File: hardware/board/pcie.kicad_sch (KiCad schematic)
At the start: 60 parts, among them CN2 1-2199230-5, U46 PI6C557-03BLE, U50 TP5108E23E-33, U51 SY8089AAAC, X6 X322525MOB4SI

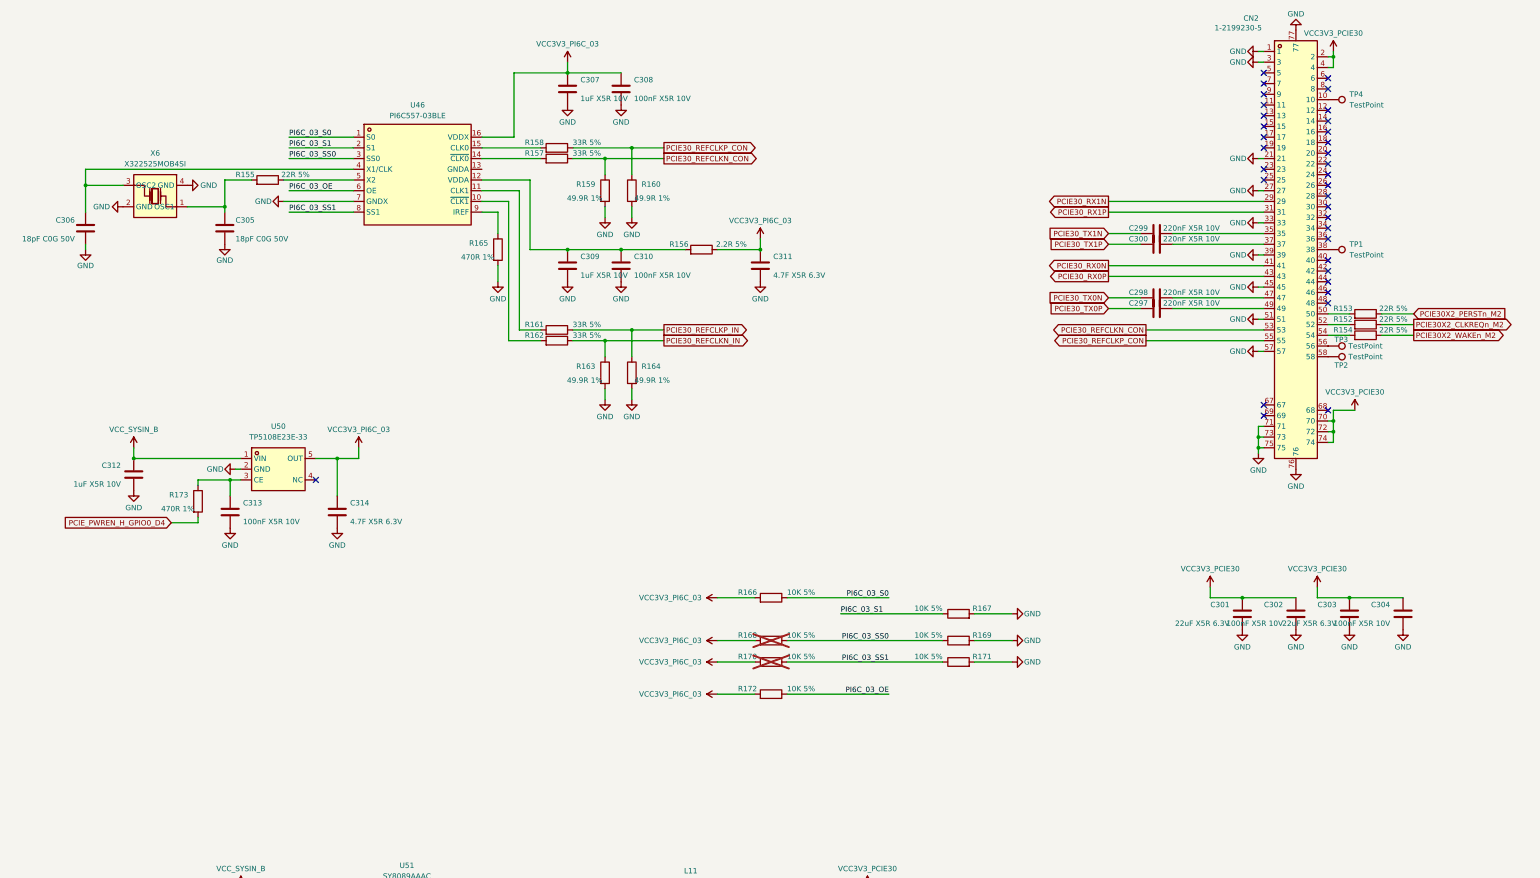
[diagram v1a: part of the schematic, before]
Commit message: finished schematic!
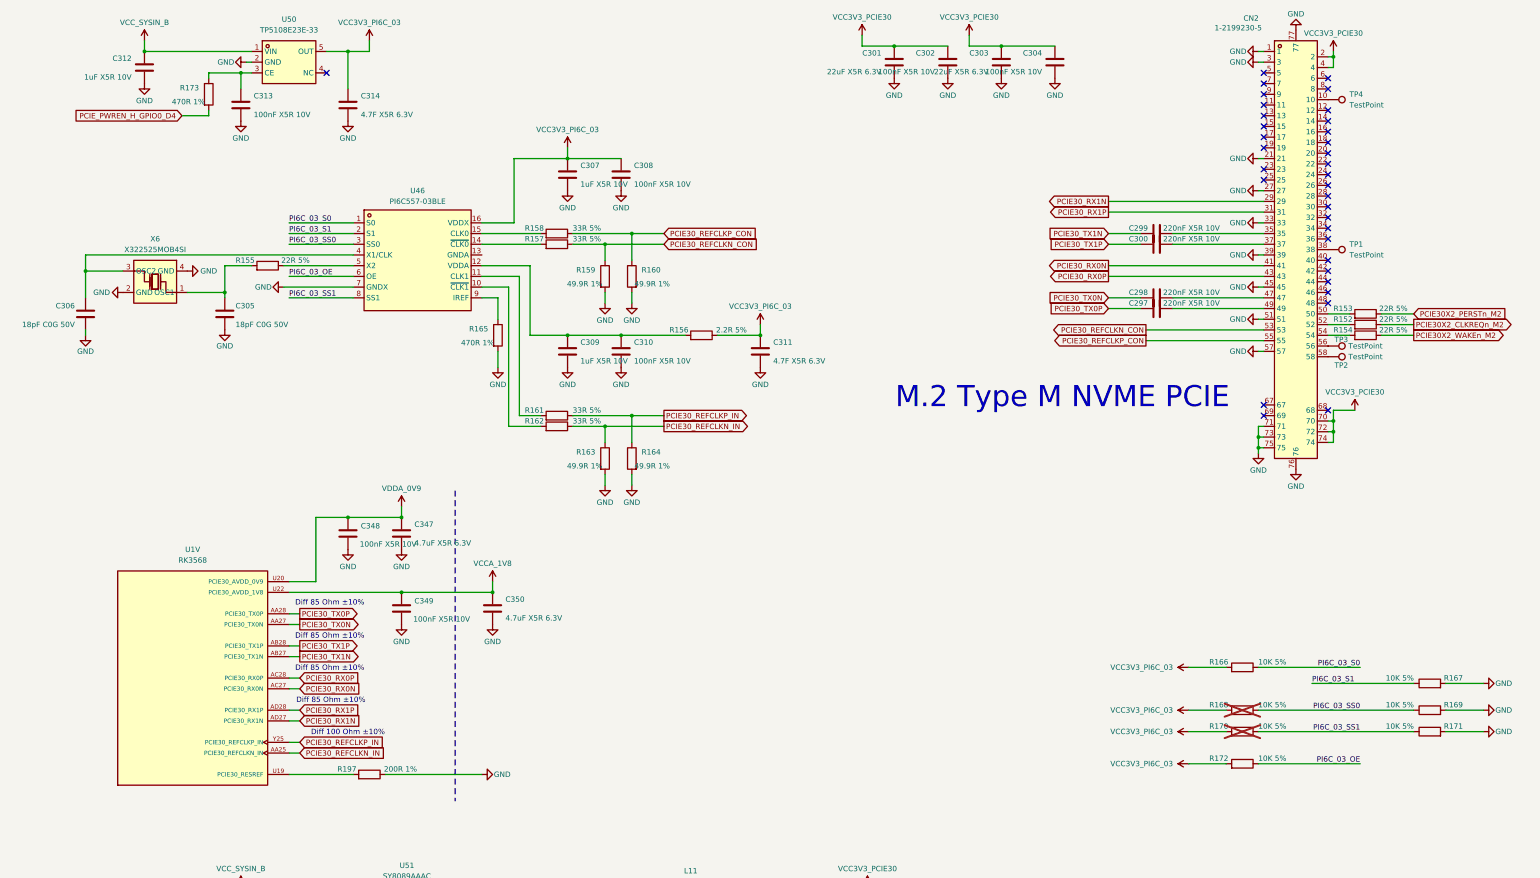
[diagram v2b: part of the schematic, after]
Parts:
- added C347, C350: 4.7uF X5R 6.3V, Capacitor_SMD:C_0402_1005Metric, symbol Device:C
- added C348, C349: 100nF X5R 10V, Capacitor_SMD:C_0201_0603Metric, symbol Device:C
- added R197: 200R 1%, Resistor_SMD:R_0201_0603Metric, symbol Device:R
- added U1: RK3568, RK3568:BGA636C65P28X28_1900X1900X168, symbol RK3568:RK3568
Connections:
- net GND: now also C347.2, C348.2, C349.2, C350.2, R197.1
- net PCIE30_REFCLKN_IN: now also U1.AA25 (PCIE30_REFCLKN_IN)
- net PCIE30_REFCLKP_IN: now also U1.Y25 (PCIE30_REFCLKP_IN)
- net PCIE30_RX0N: now also U1.AC27 (PCIE30_RX0N)
- net PCIE30_RX0P: now also U1.AC28 (PCIE30_RX0P)
- net PCIE30_RX1N: now also U1.AD27 (PCIE30_RX1N)
- net PCIE30_RX1P: now also U1.AD28 (PCIE30_RX1P)
- net PCIE30_TX0N: now also U1.AA27 (PCIE30_TX0N)
- net PCIE30_TX0P: now also U1.AA28 (PCIE30_TX0P)
- net PCIE30_TX1N: now also U1.AB27 (PCIE30_TX1N)
- net PCIE30_TX1P: now also U1.AB28 (PCIE30_TX1P)
- new net: R197.2, U1.U19 (PCIE30_RESREF)
- new net PCIE30_AVDD_0V9: C347.1, C348.1, U1.U20 (PCIE30_AVDD_0V9), U1.U21 (PCIE30_AVDD_0V9)
- new net VCCA_1V8: C349.1, C350.1, U1.U22 (PCIE30_AVDD_1V8)
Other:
- note added: "Diff 100 Ohm ±10%"
- note added: "Diff 85 Ohm ±10%"
- note added: "M.2 Type M NVME PCIE"
- moved on the sheet: C301, C302, C303, C304, C305, C306, C307, C308, C309, C310, C311, C312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

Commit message: finished beautifying schematic
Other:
- note added: "Clock Generator"
- note added: "Frost"
- note added: "M.2 Type B"
- note added: "Power / Decoupling"
- note added: "RK3568"
- note removed: "M.2 Type M NVME PCIE"
- moved on the sheet: C301, C302, C303, C304, C305, C306, C307, C308, C309, C310, C311, C312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

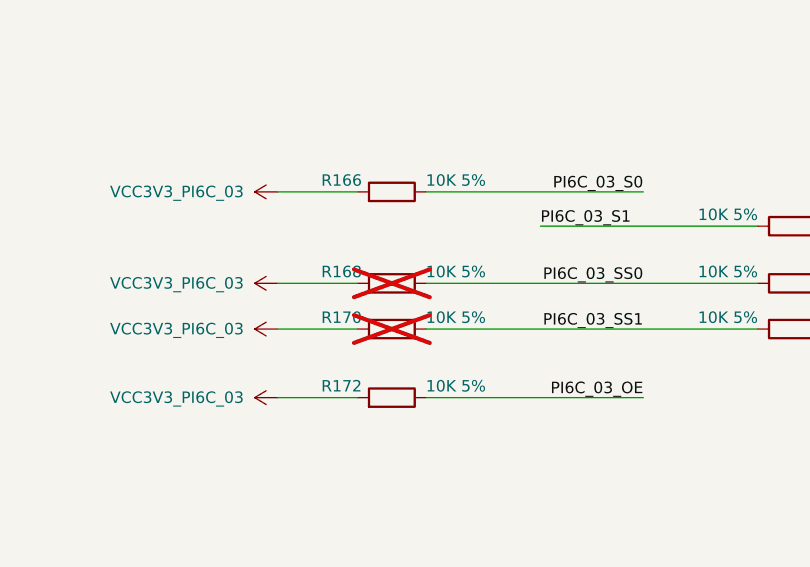
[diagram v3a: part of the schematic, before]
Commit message: did a thing
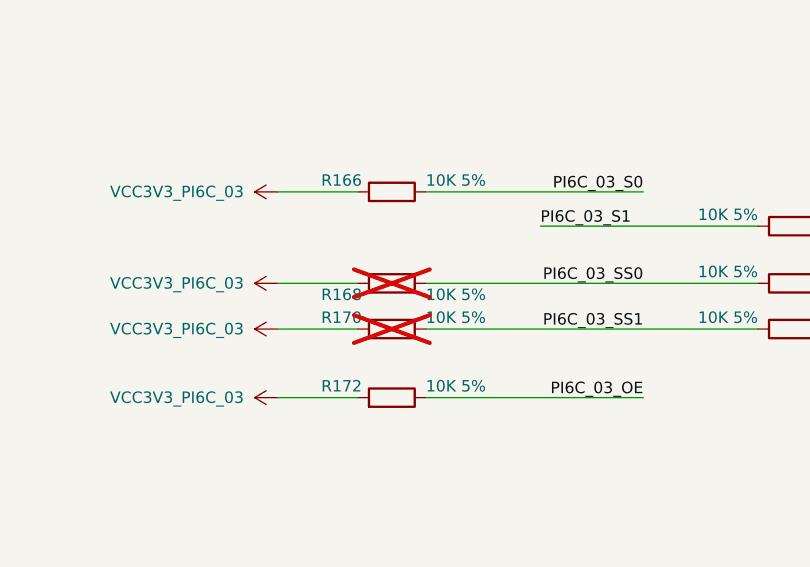
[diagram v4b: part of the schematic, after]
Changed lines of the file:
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@@
 		(exclude_from_sim no)
 		(in_bom yes)
-		(on_board yes)
+		(on_board no)
 		(dnp yes)
 		(property "Reference" "R170"
@@
 		(lib_id "Device:R")
 		(at 95.25 119.38 270)
-		(mirror x)
 		(unit 1)
 		(exclude_from_sim no)
 		(in_bom yes)
-		(on_board yes)
+		(on_board no)
 		(dnp yes)
 		(property "Reference" "R168"
-			(at 89.662 118.11 90)
+			(at 89.662 120.65 90)
 			(effects
 				(font
@@
 		)
 		(property "Value" "10K 5%"
-			(at 102.362 118.11 90)
+			(at 102.362 120.65 90)
 			(effects
 				(font
@@
 		)
 		(property "Footprint" "Resistor_SMD:R_0402_1005Metric"
-			(at 95.25 121.158 90)
+			(at 95.25 117.602 90)
 			(effects
 				(font
